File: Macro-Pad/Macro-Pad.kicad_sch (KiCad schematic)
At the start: 1 part, among them U1 ESP32-S3-WROOM-1

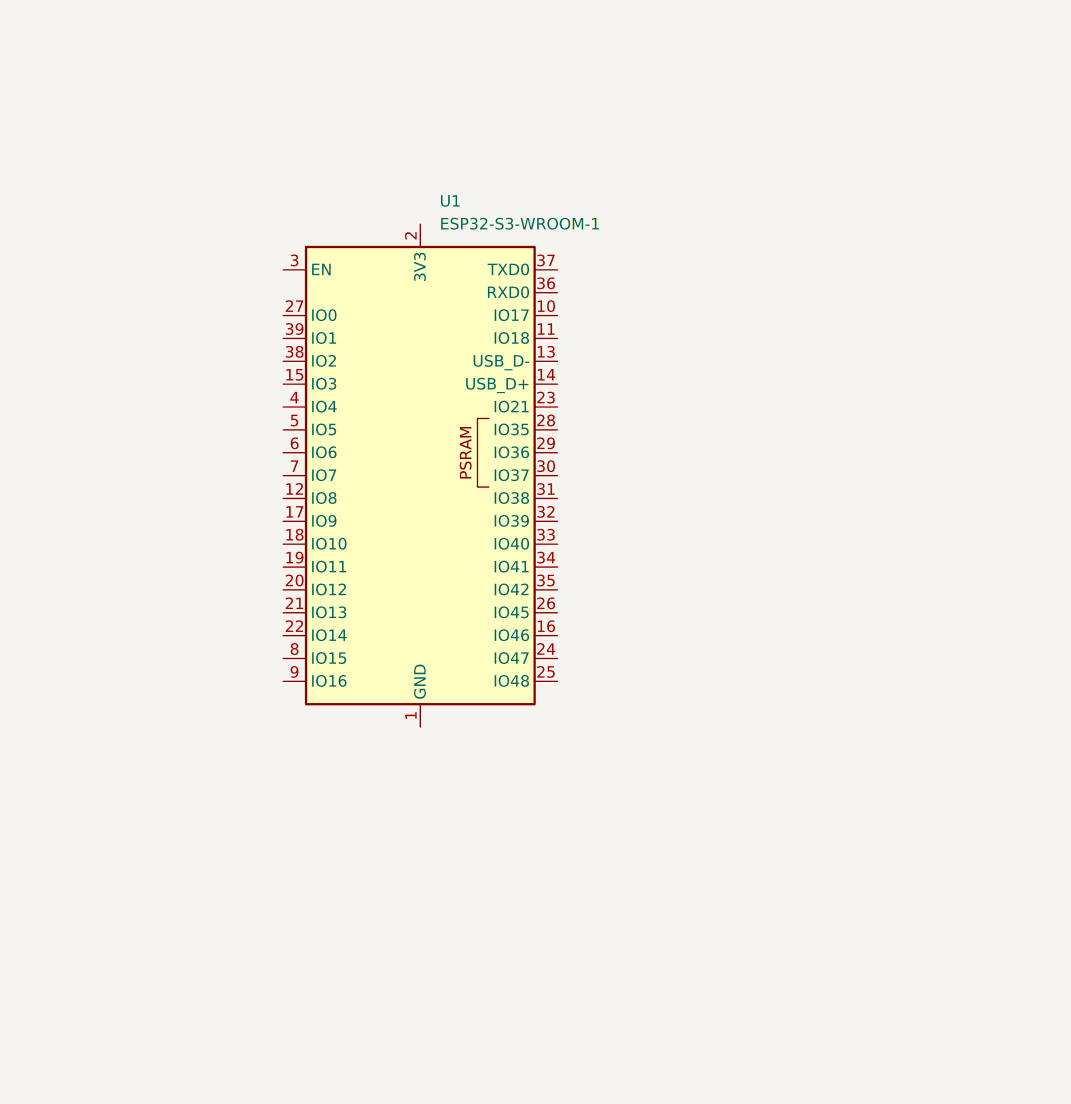
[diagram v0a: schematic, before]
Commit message: v1
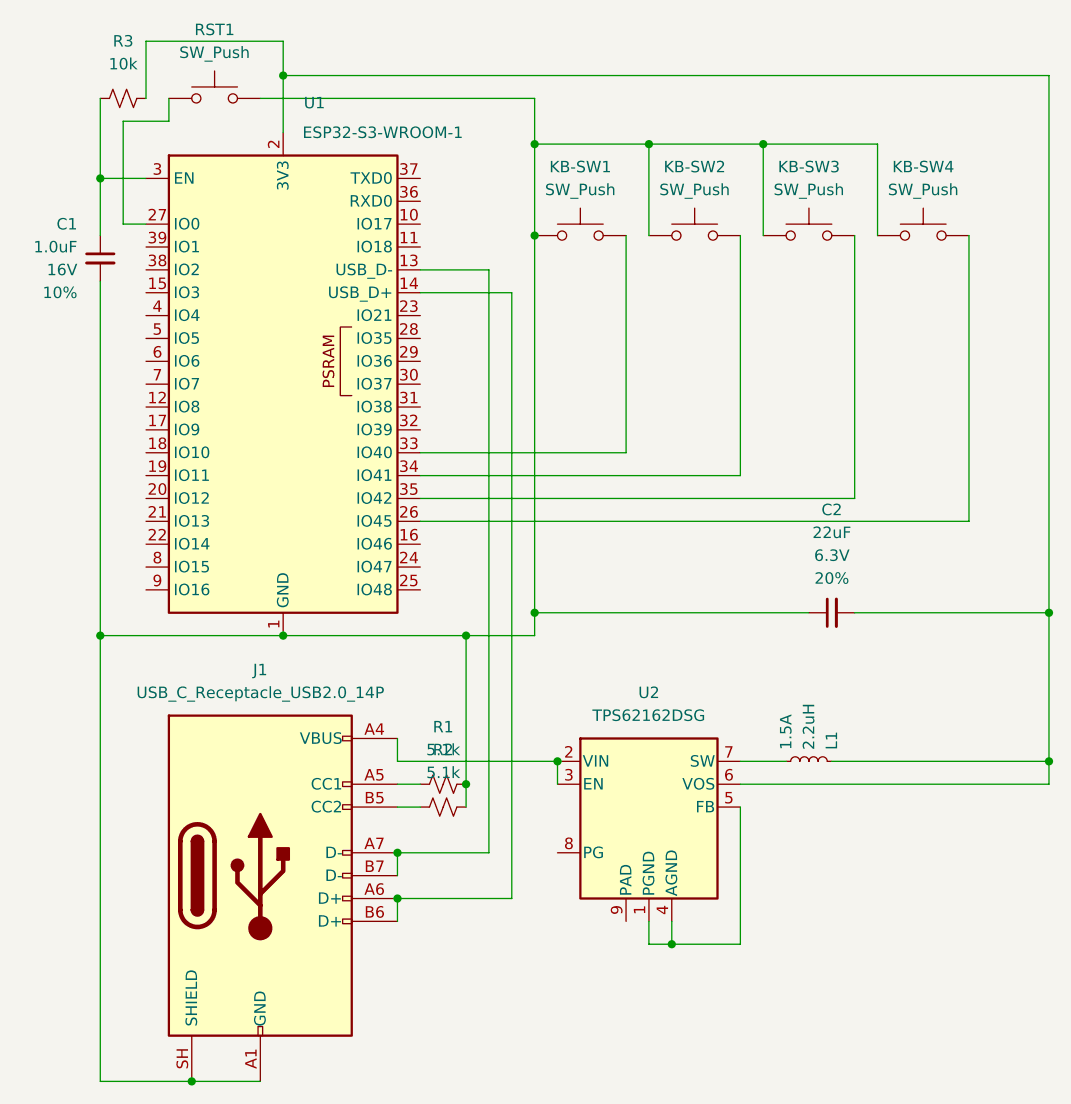
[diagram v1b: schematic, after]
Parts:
- added C1: 1.0uF, PCM_SparkFun-Capacitor:C_0402_1005Metric, symbol PCM_SparkFun-Capacitor:1.0uF_0402_16V_10%
- added C2: 22uF, PCM_SparkFun-Capacitor:C_0402_1005Metric, symbol PCM_SparkFun-Capacitor:10uF_0402_6.3V_20%
- added J1: USB_C_Receptacle_USB2.0_14P, Connector_USB:USB_C_Receptacle_HRO_TYPE-C-31-M-12, symbol Connector:USB_C_Receptacle_USB2.0_14P
- added KB-SW1, KB-SW2, KB-SW3, KB-SW4: SW_Push, Button_Switch_Keyboard:SW_Cherry_MX_1.00u_PCB, symbol Switch:SW_Push
- added L1: 2.2uH, PCM_SparkFun-Coil:0806, symbol PCM_SparkFun-Coil:2.2uH_0806_1.2A
- added R1, R2: 5.1k, PCM_SparkFun-Resistor:R_0603_1608Metric, symbol PCM_SparkFun-Resistor:5.1k_0603
- added R3: 10k, PCM_SparkFun-Resistor:R_0603_1608Metric, symbol PCM_SparkFun-Resistor:10k_0603
- added RST1: SW_Push, Button_Switch_SMD:SW_SPST_PTS645Sx43SMTR92, symbol Switch:SW_Push
- added U2: TPS62162DSG, Package_SON:Texas_DSG0008A_WSON-8-1EP_2x2mm_P0.5mm_EP0.9x1.6mm_ThermalVias, symbol Regulator_Switching:TPS62162DSG
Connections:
- net at U1.1 (GND), U1.40 (GND), U1.41 (GND): now also C1.2, C2.1, J1.A1 (GND), J1.A12 (GND), J1.B1 (GND), J1.B12 (GND), J1.SH (SHIELD), KB-SW1.1, KB-SW2.1, KB-SW3.1, KB-SW4.1, R1.2, R2.2, RST1.2
- net at U1.13 (USB_D-): now also J1.A7 (D-), J1.B7 (D-)
- net at U1.14 (USB_D+): now also J1.A6 (D+), J1.B6 (D+)
- net at U1.2 (3V3): now also C2.2, L1.1, R3.2, U2.6 (VOS)
- net at U1.26 (IO45): now also KB-SW4.2
- net at U1.27 (IO0): now also RST1.1
- net at U1.3 (EN): now also C1.1, R3.1
- net at U1.33 (IO40): now also KB-SW1.2
- net at U1.34 (IO41): now also KB-SW2.2
- net at U1.35 (IO42): now also KB-SW3.2
- new net: U2.1 (PGND), U2.4 (AGND), U2.5 (FB)
- new net: J1.A4 (VBUS), J1.A9 (VBUS), J1.B4 (VBUS), J1.B9 (VBUS), U2.2 (VIN), U2.3 (EN)
- new net: L1.2, U2.7 (SW)
- new net: J1.B5 (CC2), R2.1
- new net: J1.A5 (CC1), R1.1
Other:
- moved on the sheet: U1
